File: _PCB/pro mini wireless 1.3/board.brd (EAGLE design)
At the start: 34.1 x 61.4 mm, 14 parts

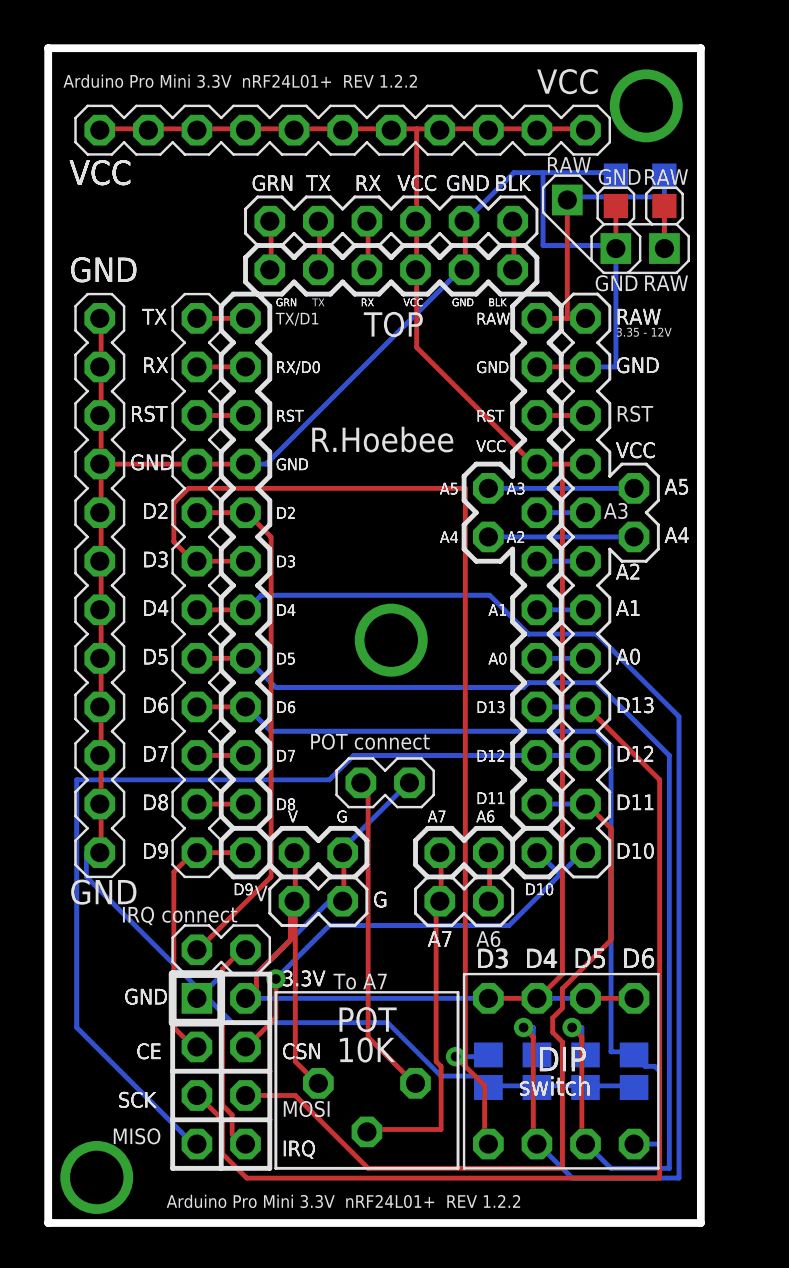
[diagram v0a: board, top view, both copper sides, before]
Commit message: update
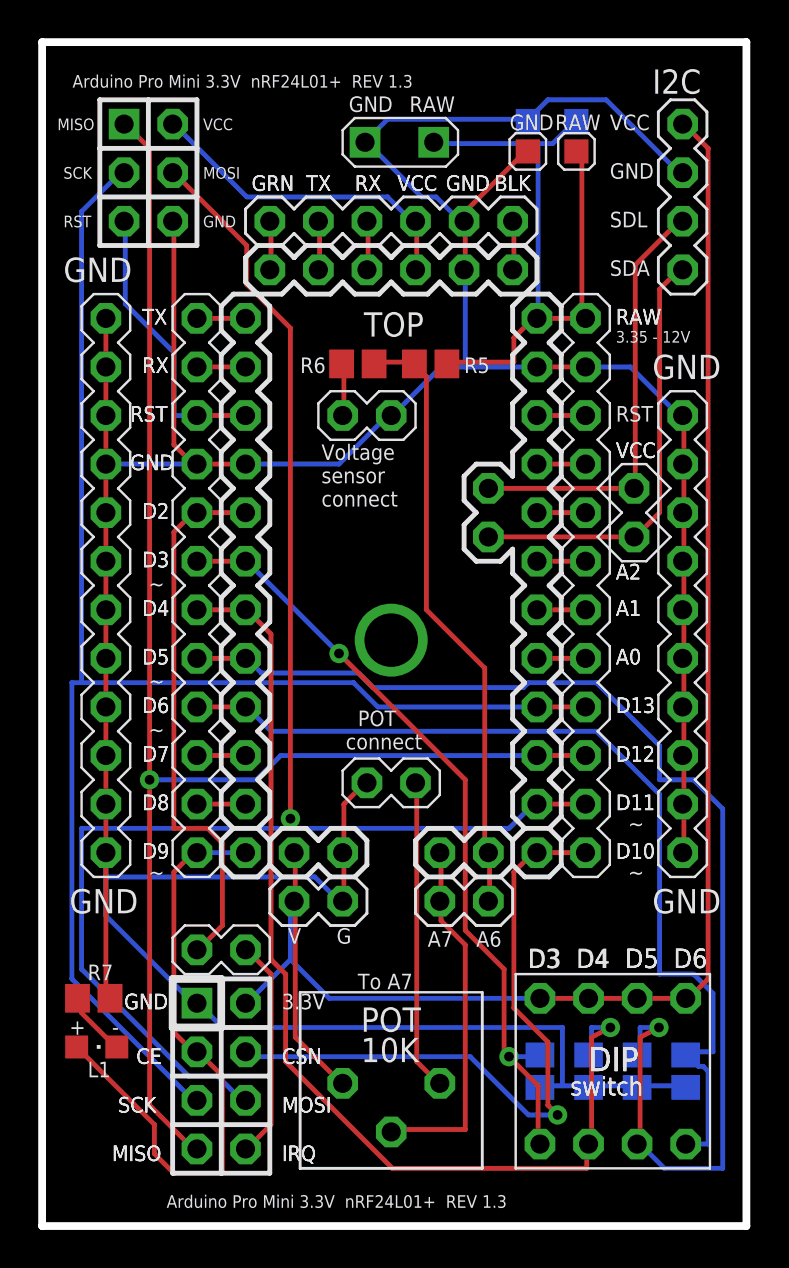
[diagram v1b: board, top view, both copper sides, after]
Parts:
- added U$15, U$20: 2_PIN_HEADER, 2_PIN_HEADER:2_PIN_HEADER
- added U$16, U$17: 1k, 0805_SMD:0805_SMD_RESISTOR
- added U$18: 0805_SMD_LED, 0805_SMD:0805_SMD_LED
- added U$19: ???R, 0805_SMD:0805_SMD_RESISTOR
- added U$21: NRF24L01, nrf24l01_connection:NRFL2401
- added U$22: SCREWTERMINAL, 18650_batt_connect:SCREWTERMINAL
- added U$23: SPI, SPI:SPI
- U$11: value (none) -> 4_PIN_HEADER; device DIPS_Arduino:4-DIP -> Headers:4_PIN_HEADER
- U$12: value 18650_BATT_CONECT -> 10_PIN_HEADER; device 18650_batt_connect:18650_BATT_CONECT -> Headers:10_PIN_HEADER
- U$3: value 12_2_HEADER -> (none); device 12_2_HEADER:12_2_HEADER -> 12_pin_header:12_PIN_HEADER
- U$4: value NRF2L01-3 -> PAD_CONNECT; device nrf24l01_connection:NRF24L01-3 -> 18650_batt_connect:PAD_CONNECT
- U$8: value (none) -> 12_PIN_HEADER; device 12_pin_header:12_PIN_HEADER -> Headers:12_PIN_HEADER
- U$9: value 11_PIN_HEADER -> (none); device 11_pin_header:11_PIN_HEADER -> DIPS_Arduino:4-DIP
- moved U$4 51.3 mm to (58.9, 61.1)
- moved U$9 51.3 mm to (62.1, 13.0), turned to 0 degrees
- moved U$11 45.8 mm to (65.7, 58.4), turned to 270 degrees
- moved U$12 13.9 mm to (65.7, 35.6)
- moved U$14 4.32 mm to (50.5, 27.8)
- moved U$10 4.02 mm to (41.6, 19.1)
- moved U$3 3.59 mm to (60.6, 39.4)
- moved U$8 1.31 mm to (35.6, 38.1)
- moved U$13 1.27 mm to (50.5, 12.4)
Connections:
- removed net N$12: U$1.D9, U$2.12, U$4.CE
- removed net N$22: U$1.A5, U$3.13
- removed net N$33: U$1.A6, U$6.4
- new net N$21: U$1.A4, U$11.4, U$20.2
- new net N$24: U$1.D9, U$18.A, U$2.12, U$21.CE
- new net N$27: U$1.RAW, U$17.2, U$22.RAW_3, U$3.1, U$4.RAW_1, U$4.RAW_2
- new net N$35: U$1.D6, U$2.9, U$9.D6, U$9.OFF_4
- new net N$7: U$1.A5, U$11.3, U$20.1
- new net N$8: U$1.VCC_1, U$23.VCC, U$5.4
- new net N$9: U$15.2, U$16.1
- net GND: now also U$11.2, U$12.P$1, U$12.P$10, U$12.P$2, U$12.P$3, U$12.P$4, U$12.P$5, U$12.P$6, U$12.P$7, U$12.P$8, U$12.P$9, U$14.2, U$15.1, U$19.2, U$21.GND, U$22.GND, U$23.GND, U$4.GND_1, U$4.GND_2, U$9.GND_1, U$9.GND_2, U$9.GND_3, U$9.GND_4; no longer U$11.GND_1, U$11.GND_2, U$11.GND_3, U$11.GND_4, U$12.GND, U$12.GND_1, U$12.GND_2, U$14.1, U$4.GND
- net N$10: now also U$14.1; no longer U$14.2
- net N$11: now also U$18.C, U$19.1; no longer U$1.D4, U$11.D4, U$11.OFF_2, U$2.7
- net N$13: now also U$21.CSN; no longer U$4.CSN
- net N$14: now also U$21.MOSI, U$23.MOSI; no longer U$4.MOSI
- net N$15: now also U$1.D3, U$2.6, U$9.D3, U$9.OFF_1; no longer U$1.D12, U$3.10, U$4.MISO
- net N$23: now also U$1.A6, U$16.2, U$17.1, U$6.4; no longer U$1.A4, U$3.14
- net N$28: now also U$1.D12, U$21.MISO, U$23.MISO, U$3.10; no longer U$1.D3, U$11.D3, U$11.OFF_1, U$2.6
- net N$29: now also U$9.D5, U$9.OFF_3; no longer U$11.D5, U$11.OFF_3
- net N$3: now also U$23.RESET
- net N$30: now also U$1.D4, U$2.7, U$9.D4, U$9.OFF_2; no longer U$1.D6, U$11.D6, U$11.OFF_4, U$2.9
- net N$37: now also U$21.SCK, U$23.SCK; no longer U$4.SCK
- net N$5: now also U$21.IRQ; no longer U$4.IRQ
- net N$6: now also U$1.VCC_0, U$3.4; no longer U$1.RAW, U$12.RAW, U$12.RAW_1, U$12.RAW_2, U$12.RAW_3, U$3.1
- net VCC: now also U$11.1, U$21.3.3V, U$9.VCC_1, U$9.VCC_2, U$9.VCC_3, U$9.VCC_4; no longer U$1.VCC_0, U$1.VCC_1, U$11.VCC_1, U$11.VCC_2, U$11.VCC_3, U$11.VCC_4, U$3.4, U$4.3.3V, U$5.4, U$9.P$1, U$9.P$10, U$9.P$11, U$9.P$2, U$9.P$3, U$9.P$4, U$9.P$5, U$9.P$6, U$9.P$7, U$9.P$8, U$9.P$9
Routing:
- net GND: track 137.6 -> 205.1 mm
- net N$11: track 69.0 -> 3.56 mm, vias 1 -> 0
- net N$35: track 0.00 -> 49.7 mm
- net N$14: track 41.8 -> 82.5 mm, vias 0 -> 1
- net N$27: track 0.00 -> 35.0 mm
- net N$24: track 0.00 -> 32.4 mm
- net VCC: track 116.5 -> 88.2 mm
- net N$23: track 7.62 -> 32.1 mm
- net N$37: track 55.8 -> 79.8 mm
- net N$7: track 0.00 -> 22.8 mm, vias 1 -> 0
- net N$21: track 0.00 -> 22.8 mm
- net N$28: track 59.1 -> 78.6 mm
- net N$8: track 0.00 -> 17.5 mm, vias 1 -> 0
- net N$6: track 20.0 -> 2.54 mm
- net N$12: track 13.9 -> 0.00 mm
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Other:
- board size 34.1 x 61.4 mm -> 36.8 x 61.9 mm
- board text added: "+"
- board text added: "-"
- board text added: "Arduino Pro Mini 3.3V nRF24L01+ REV 1.3"
- board text added: "I2C"
- board text added: "L1"
- board text added: "R1"
- board text added: "R2"
- board text added: "R3"
- board text added: "R4"
- board text added: "R5"
- board text added: "R6"
- board text added: "R7"
- board text added: "SDA"
- board text added: "SDL"
- board text added: "Voltage sensor connect"
- board text added: "~"
- board text removed: "A3"
- board text removed: "A4"
- board text removed: "A5"
- board text removed: "Arduino Pro Mini 3.3V nRF24L01+ REV 1.2.2"
- board text removed: "IRQ connect"
- board text removed: "R.Hoebee"
